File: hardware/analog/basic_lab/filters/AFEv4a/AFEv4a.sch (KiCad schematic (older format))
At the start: 2 parts

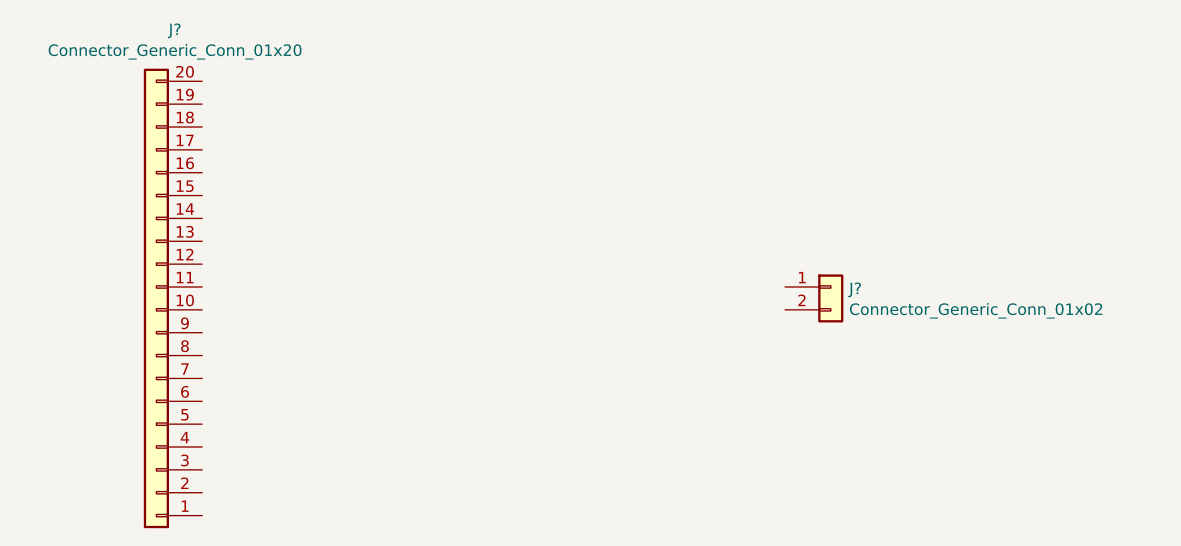
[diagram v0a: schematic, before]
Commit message: ice40qfn restarted: simplest design ready?
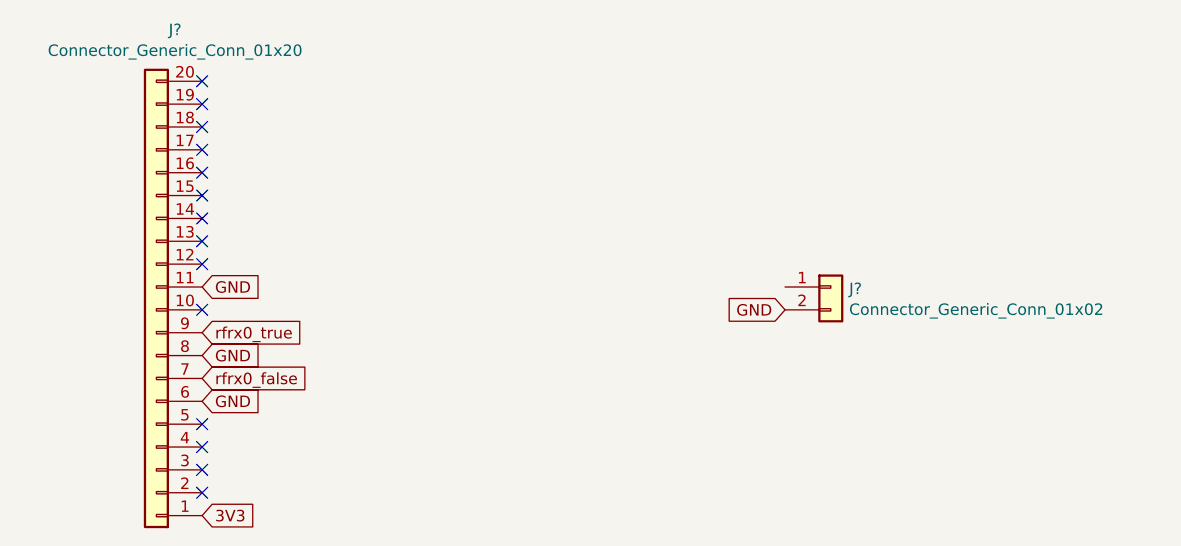
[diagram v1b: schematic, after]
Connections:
- net 3V3: now reaches J?.1 (Pin_1)
- net GND: now reaches J?.11 (Pin_11)
- net GND: now also J?.2 (Pin_2), J?.6 (Pin_6), J?.8 (Pin_8)
- net rfrx0_false: now reaches J?.7 (Pin_7)
- net rfrx0_true: now reaches J?.9 (Pin_9)
- no-connect marks 0 -> 14
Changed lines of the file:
@@
 	1    0    0    -1
 $EndComp
+Text GLabel 1800 3350 2    50   Input ~ 0
+rfrx0_true
+Text GLabel 1800 3550 2    50   Input ~ 0
+rfrx0_false
+Text GLabel 1800 4150 2    50   Input ~ 0
+3V3
+Text GLabel 1800 3150 2    50   Input ~ 0
+GND
+Text GLabel 1800 3450 2    50   Input ~ 0
+GND
+Text GLabel 1800 3650 2    50   Input ~ 0
+GND
+NoConn ~ 1800 4050
+NoConn ~ 1800 3950
+NoConn ~ 1800 3850
+NoConn ~ 1800 3750
+NoConn ~ 1800 3250
+NoConn ~ 1800 3050
+NoConn ~ 1800 2250
+NoConn ~ 1800 2350
+NoConn ~ 1800 2450
+NoConn ~ 1800 2550
+NoConn ~ 1800 2650
+NoConn ~ 1800 2750
+NoConn ~ 1800 2850
+NoConn ~ 1800 2950
+Text GLabel 4350 3250 0    50   Input ~ 0
+GND
 $EndSCHEMATC
